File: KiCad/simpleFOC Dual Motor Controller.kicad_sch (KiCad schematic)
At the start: 15 parts, among them J101 Conn_02x03_Counter_Clockwise, U101 STM32F103C8Tx, U102 XT60H-M

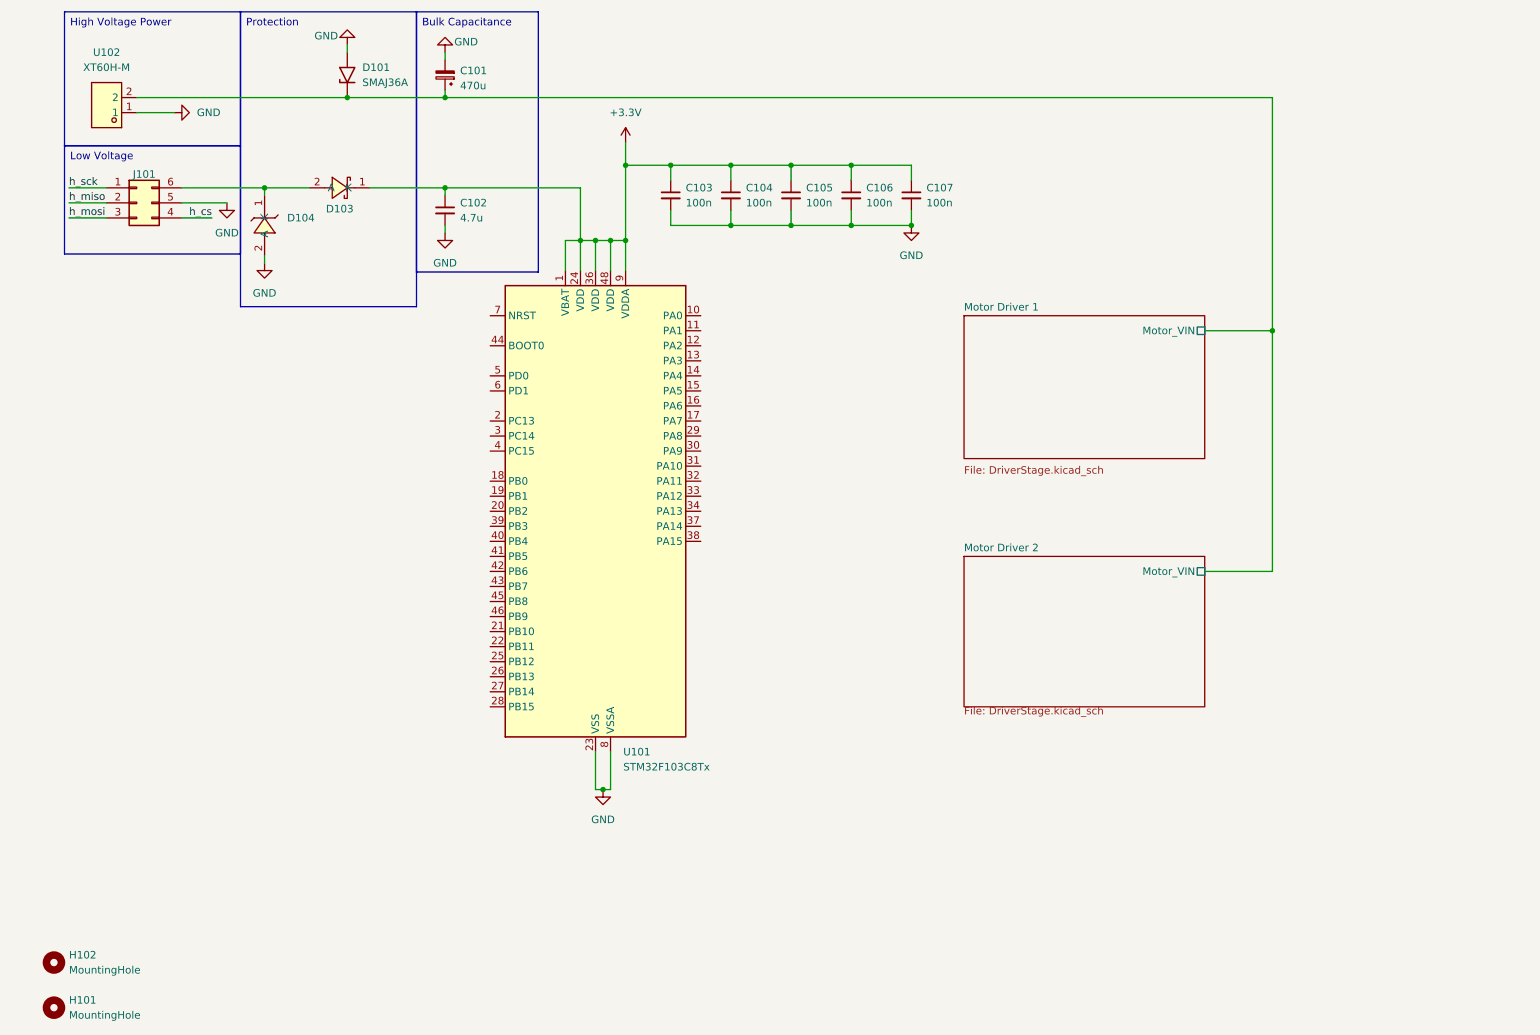
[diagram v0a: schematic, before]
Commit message: start adding control pins
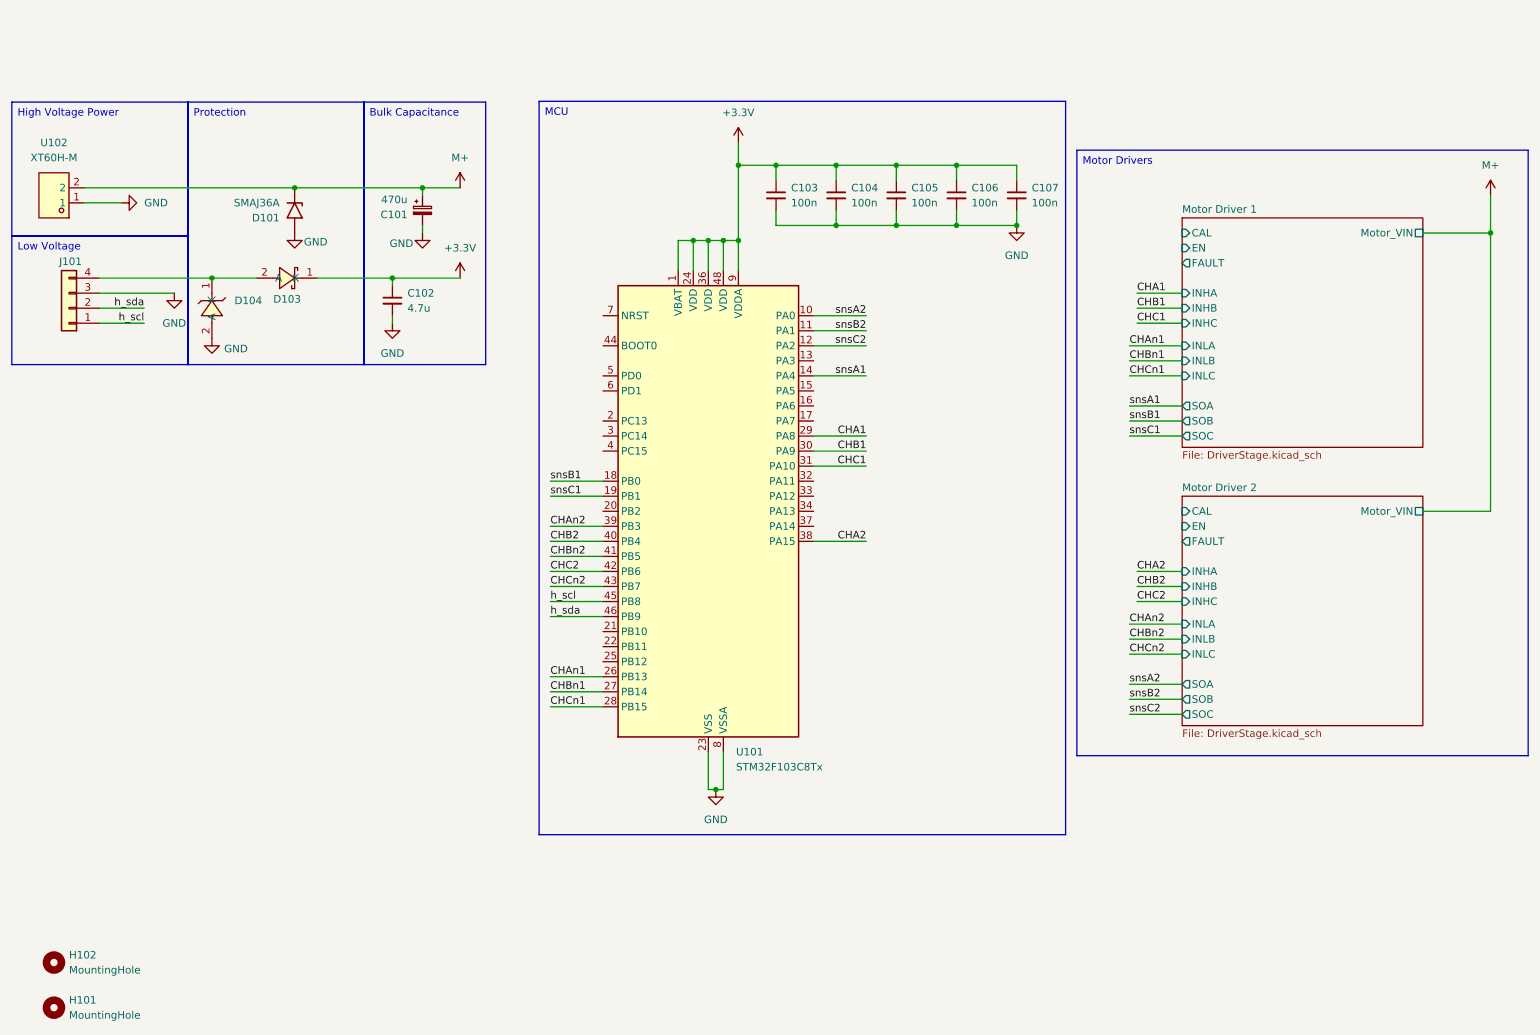
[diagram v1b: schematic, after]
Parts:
- removed J101: Conn_02x03_Counter_Clockwise, symbol Connector_Generic:Conn_02x03_Counter_Clockwise
- added J101: Conn_01x04, PCM_SparkFun-Connector:JST_1x04_P2.0mm_Vertical_PTH, symbol PCM_SparkFun-Connector:Conn_01x04_JST_P2.0mm_Vertical_PTH
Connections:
- net GND: now also J101.3 (Pin_3)
- net at D103.2 (A), D104.1 (K): now also J101.4 (Pin_4)
- net snsA2: now reaches U101.10 (PA0)
- net snsB2: now reaches U101.11 (PA1)
- net snsC2: now reaches U101.12 (PA2)
- net snsA1: now reaches U101.14 (PA4)
- net snsB1: now reaches U101.18 (PB0)
- net snsC1: now reaches U101.19 (PB1)
- net CHAn1: now reaches U101.26 (PB13)
- net CHBn1: now reaches U101.27 (PB14)
- net CHCn1: now reaches U101.28 (PB15)
- net CHA1: now reaches U101.29 (PA8)
- net CHB1: now reaches U101.30 (PA9)
- net CHC1: now reaches U101.31 (PA10)
- net CHA2: now reaches U101.38 (PA15)
- net CHAn2: now reaches U101.39 (PB3)
- net CHB2: now reaches U101.40 (PB4)
- net CHBn2: now reaches U101.41 (PB5)
- net CHC2: now reaches U101.42 (PB6)
- net CHCn2: now reaches U101.43 (PB7)
- net h_scl: now reaches U101.45 (PB8)
- net h_scl: now also J101.1 (Pin_1)
- net h_sda: now reaches U101.46 (PB9)
- net h_sda: now also J101.2 (Pin_2)
- net Motor Driver 1/Motor_VIN renamed M+
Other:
- sheet Motor Driver 1 ports: added CAL, EN, FAULT, INHA, INHB, INHC, INLA, INLB, INLC, SOA, SOB, SOC; removed none
- sheet Motor Driver 2 ports: added CAL, EN, FAULT, INHA, INHB, INHC, INLA, INLB, INLC, SOA, SOB, SOC; removed none
- moved on the sheet: C101, C102, C103, C104, C105, C106, C107, D101, D103, D104, U101, U102
